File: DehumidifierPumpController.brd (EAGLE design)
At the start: 68.6 x 53.3 mm, 6 parts, among them P1 12V

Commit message: updated Picture and tinkercad sketch file
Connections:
- removed net N$4 (its old number): R4.2, U1.GND.
- removed net N$9 (its old number): K1.1, U1.GND
- new net N$2: K1.1, R4.2, U1.GND.
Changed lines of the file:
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@@
 <element value="" name="U1" library="AUTODESK_CIRCUITS_BREADBOARD" package="ARDUINO_UNO" x="5" y="10.08"></element><element value="" name="S1" library="AUTODESK_CIRCUITS_BREADBOARD" package="TL1105" x="5" y="22.78"></element><element value="" name="M1" library="AUTODESK_CIRCUITS_BREADBOARD" package="2P-2.54-65/35MIL" x="5" y="35.480000000000004"></element><element value="" name="K1" library="AUTODESK_CIRCUITS_BREADBOARD" package="M3XXH" x="5" y="48.18"></element><element value="1k‎Ω" name="R4" library="AUTODESK_CIRCUITS_BREADBOARD" package="0207/10" x="5" y="60.879999999999995"></element><element value="12V" name="P1" library="AUTODESK_CIRCUITS_BREADBOARD" package="2P-2.54-65/35MIL" x="5" y="73.58"></element></elements>
 <signals>
-<signal name="N$1"><contactref element="S1" pad="4"></contactref><contactref element="R4" pad="1"></contactref><wire x1="7.25" y1="19.53" x2="-0.08000000000000007" y2="60.879999999999995" width="0" layer="19" extent="1-1"></wire></signal><signal name="N$2"><contactref element="S1" pad="2"></contactref><contactref element="U1" pad="2"></contactref><wire x1="7.25" y1="26.03" x2="63.42" y2="60.879999999999995" width="0" layer="19" extent="1-1"></wire></signal><signal name="N$3"><contactref element="S1" pad="1"></contactref></signal><signal name="N$4"><contactref element="R4" pad="2"></contactref><contactref element="U1" pad="GND."></contactref><wire x1="10.08" y1="60.879999999999995" x2="48.18" y2="12.620000000000001" width="0" layer="19" extent="1-1"></wire></signal><signal name="N$5"><contactref element="K1" pad="2"></contactref><contactref element="U1" pad="7"></contactref><wire x1="1.19" y1="44.37" x2="50.72" y2="60.879999999999995" width="0" layer="19" extent="1-1"></wire></signal><signal name="N$6"><contactref element="M1" pad="1"></contactref><contactref element="P1" pad="1"></contactref><wire x1="5" y1="36.75000000000001" x2="5" y2="74.85" width="0" layer="19" extent="1-1"></wire></signal><signal name="N$7"><contactref element="P1" pad="2"></contactref><contactref element="K1" pad="P"></contactref><wire x1="5" y1="72.31" x2="11.35" y2="44.37" width="0" layer="19" extent="1-1"></wire></signal><signal name="N$8"><contactref element="K1" pad="S"></contactref><contactref element="M1" pad="2"></contactref><wire x1="-1.3499999999999996" y1="51.99" x2="5" y2="34.21" width="0" layer="19" extent="1-1"></wire></signal><signal name="N$9"><contactref element="U1" pad="GND"></contactref><contactref element="K1" pad="1"></contactref><wire x1="31.416" y1="60.879999999999995" x2="1.19" y2="51.99" width="0" layer="19" extent="1-1"></wire></signal><signal name="N$10"><contactref element="U1" pad="5V"></contactref><contactref element="S1" pad="3"></contactref><wire x1="43.1" y1="12.620000000000001" x2="2.75" y2="19.53" width="0" layer="19" extent="1-1"></wire></signal></signals>
+<signal name="N$1"><contactref element="S1" pad="4"></contactref><contactref element="R4" pad="1"></contactref><wire x1="7.25" y1="19.53" x2="-0.08000000000000007" y2="60.879999999999995" width="0" layer="19" extent="1-1"></wire></signal><signal name="N$2"><contactref element="U1" pad="GND."></contactref><contactref element="K1" pad="1"></contactref><wire x1="48.18" y1="12.620000000000001" x2="1.19" y2="51.99" width="0" layer="19" extent="1-1"></wire><contactref element="R4" pad="2"></contactref><wire x1="1.19" y1="51.99" x2="10.08" y2="60.879999999999995" width="0" layer="19" extent="1-1"></wire></signal><signal name="N$3"><contactref element="M1" pad="1"></contactref><contactref element="P1" pad="1"></contactref><wire x1="5" y1="36.75000000000001" x2="5" y2="74.85" width="0" layer="19" extent="1-1"></wire></signal><signal name="N$4"><contactref element="U1" pad="5V"></contactref><contactref element="S1" pad="3"></contactref><wire x1="43.1" y1="12.620000000000001" x2="2.75" y2="19.53" width="0" layer="19" extent="1-1"></wire></signal><signal name="N$5"><contactref element="U1" pad="2"></contactref><contactref element="S1" pad="2"></contactref><wire x1="63.42" y1="60.879999999999995" x2="7.25" y2="26.03" width="0" layer="19" extent="1-1"></wire></signal><signal name="N$6"><contactref element="S1" pad="1"></contactref></signal><signal name="N$7"><contactref element="K1" pad="P"></contactref><contactref element="P1" pad="2"></contactref><wire x1="11.35" y1="44.37" x2="5" y2="72.31" width="0" layer="19" extent="1-1"></wire></signal><signal name="N$8"><contactref element="U1" pad="7"></contactref><contactref element="K1" pad="2"></contactref><wire x1="50.72" y1="60.879999999999995" x2="1.19" y2="44.37" width="0" layer="19" extent="1-1"></wire></signal><signal name="N$9"><contactref element="K1" pad="S"></contactref><contactref element="M1" pad="2"></contactref><wire x1="-1.3499999999999996" y1="51.99" x2="5" y2="34.21" width="0" layer="19" extent="1-1"></wire></signal></signals>
 </board>
 </drawing>

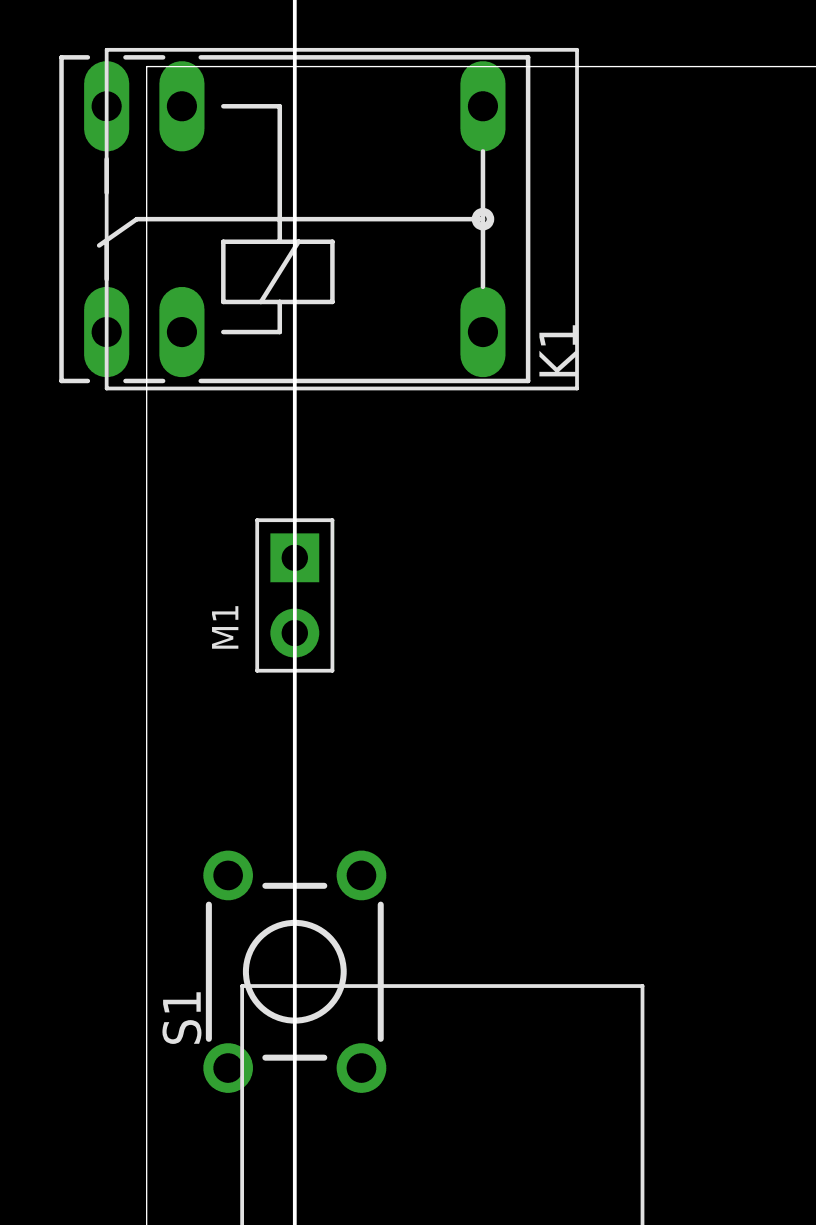
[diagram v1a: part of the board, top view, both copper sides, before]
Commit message: updated some files
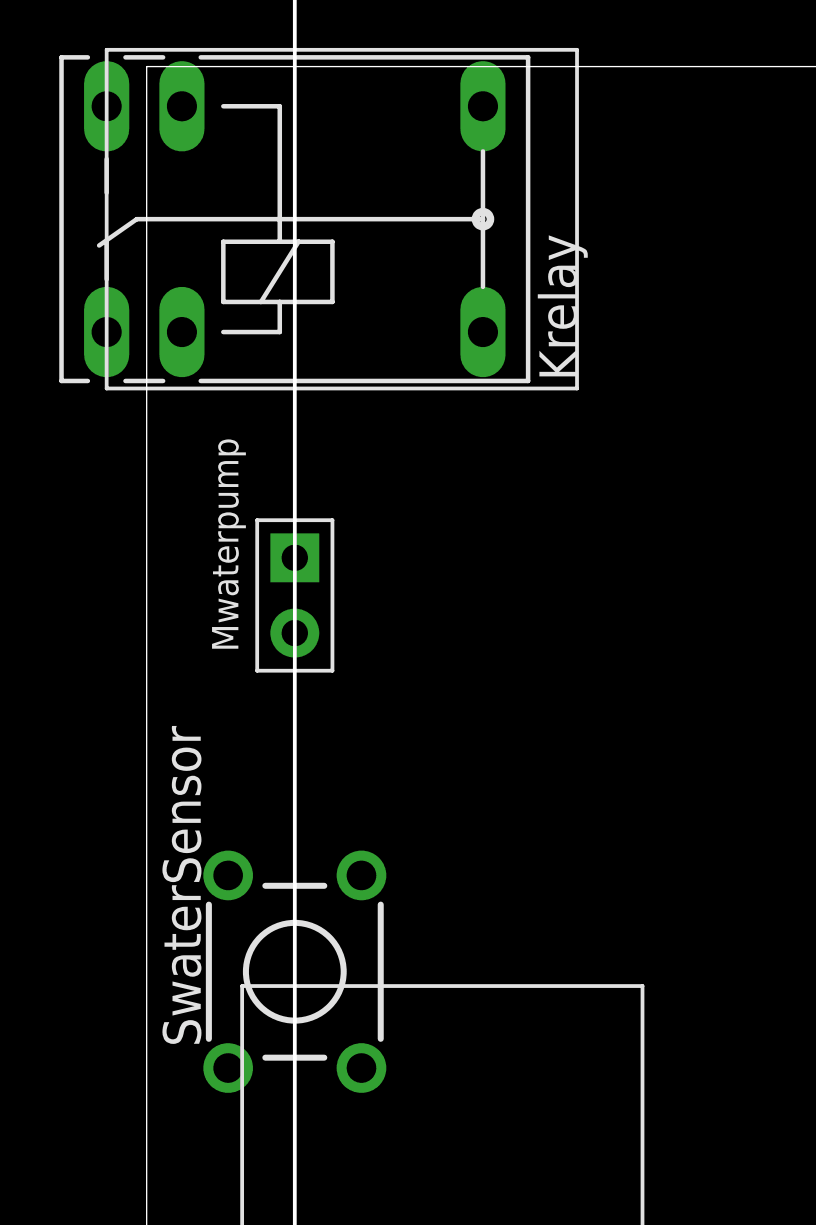
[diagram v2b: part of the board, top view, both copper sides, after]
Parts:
- renumbered K1 to Krelay, M1 to Mwaterpump, S1 to SwaterSensor
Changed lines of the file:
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@@
 </autorouter>
 <elements>
-<element value="" name="U1" library="AUTODESK_CIRCUITS_BREADBOARD" package="ARDUINO_UNO" x="5" y="10.08"></element><element value="" name="S1" library="AUTODESK_CIRCUITS_BREADBOARD" package="TL1105" x="5" y="22.78"></element><element value="" name="M1" library="AUTODESK_CIRCUITS_BREADBOARD" package="2P-2.54-65/35MIL" x="5" y="35.480000000000004"></element><element value="" name="K1" library="AUTODESK_CIRCUITS_BREADBOARD" package="M3XXH" x="5" y="48.18"></element><element value="1k‎Ω" name="R4" library="AUTODESK_CIRCUITS_BREADBOARD" package="0207/10" x="5" y="60.879999999999995"></element><element value="12V" name="P1" library="AUTODESK_CIRCUITS_BREADBOARD" package="2P-2.54-65/35MIL" x="5" y="73.58"></element></elements>
+<element value="" name="U1" library="AUTODESK_CIRCUITS_BREADBOARD" package="ARDUINO_UNO" x="5" y="10.08"></element><element value="" name="SwaterSensor" library="AUTODESK_CIRCUITS_BREADBOARD" package="TL1105" x="5" y="22.78"></element><element value="" name="Mwaterpump" library="AUTODESK_CIRCUITS_BREADBOARD" package="2P-2.54-65/35MIL" x="5" y="35.480000000000004"></element><element value="" name="Krelay" library="AUTODESK_CIRCUITS_BREADBOARD" package="M3XXH" x="5" y="48.18"></element><element value="1k‎Ω" name="R4" library="AUTODESK_CIRCUITS_BREADBOARD" package="0207/10" x="5" y="60.879999999999995"></element><element value="12V" name="P1" library="AUTODESK_CIRCUITS_BREADBOARD" package="2P-2.54-65/35MIL" x="5" y="73.58"></element></elements>
 <signals>
-<signal name="N$1"><contactref element="S1" pad="4"></contactref><contactref element="R4" pad="1"></contactref><wire x1="7.25" y1="19.53" x2="-0.08000000000000007" y2="60.879999999999995" width="0" layer="19" extent="1-1"></wire></signal><signal name="N$2"><contactref element="U1" pad="GND."></contactref><contactref element="K1" pad="1"></contactref><wire x1="48.18" y1="12.620000000000001" x2="1.19" y2="51.99" width="0" layer="19" extent="1-1"></wire><contactref element="R4" pad="2"></contactref><wire x1="1.19" y1="51.99" x2="10.08" y2="60.879999999999995" width="0" layer="19" extent="1-1"></wire></signal><signal name="N$3"><contactref element="M1" pad="1"></contactref><contactref element="P1" pad="1"></contactref><wire x1="5" y1="36.75000000000001" x2="5" y2="74.85" width="0" layer="19" extent="1-1"></wire></signal><signal name="N$4"><contactref element="U1" pad="5V"></contactref><contactref element="S1" pad="3"></contactref><wire x1="43.1" y1="12.620000000000001" x2="2.75" y2="19.53" width="0" layer="19" extent="1-1"></wire></signal><signal name="N$5"><contactref element="U1" pad="2"></contactref><contactref element="S1" pad="2"></contactref><wire x1="63.42" y1="60.879999999999995" x2="7.25" y2="26.03" width="0" layer="19" extent="1-1"></wire></signal><signal name="N$6"><contactref element="S1" pad="1"></contactref></signal><signal name="N$7"><contactref element="K1" pad="P"></contactref><contactref element="P1" pad="2"></contactref><wire x1="11.35" y1="44.37" x2="5" y2="72.31" width="0" layer="19" extent="1-1"></wire></signal><signal name="N$8"><contactref element="U1" pad="7"></contactref><contactref element="K1" pad="2"></contactref><wire x1="50.72" y1="60.879999999999995" x2="1.19" y2="44.37" width="0" layer="19" extent="1-1"></wire></signal><signal name="N$9"><contactref element="K1" pad="S"></contactref><contactref element="M1" pad="2"></contactref><wire x1="-1.3499999999999996" y1="51.99" x2="5" y2="34.21" width="0" layer="19" extent="1-1"></wire></signal></signals>
+<signal name="N$1"><contactref element="Mwaterpump" pad="1"></contactref><contactref element="P1" pad="1"></contactref><wire x1="5" y1="36.75000000000001" x2="5" y2="74.85" width="0" layer="19" extent="1-1"></wire></signal><signal name="N$2"><contactref element="U1" pad="5V"></contactref><contactref element="SwaterSensor" pad="3"></contactref><wire x1="43.1" y1="12.620000000000001" x2="2.75" y2="19.53" width="0" layer="19" extent="1-1"></wire></signal><signal name="N$3"><contactref element="Krelay" pad="P"></contactref><contactref element="P1" pad="2"></contactref><wire x1="11.35" y1="44.37" x2="5" y2="72.31" width="0" layer="19" extent="1-1"></wire></signal><signal name="N$4"><contactref element="U1" pad="7"></contactref><contactref element="Krelay" pad="2"></contactref><wire x1="50.72" y1="60.879999999999995" x2="1.19" y2="44.37" width="0" layer="19" extent="1-1"></wire></signal><signal name="N$5"><contactref element="Krelay" pad="S"></contactref><contactref element="Mwaterpump" pad="2"></contactref><wire x1="-1.3499999999999996" y1="51.99" x2="5" y2="34.21" width="0" layer="19" extent="1-1"></wire></signal><signal name="N$6"><contactref element="SwaterSensor" pad="4"></contactref><contactref element="R4" pad="1"></contactref><wire x1="7.25" y1="19.53" x2="-0.08000000000000007" y2="60.879999999999995" width="0" layer="19" extent="1-1"></wire></signal><signal name="N$7"><contactref element="SwaterSensor" pad="2"></contactref><contactref element="U1" pad="2"></contactref><wire x1="7.25" y1="26.03" x2="63.42" y2="60.879999999999995" width="0" layer="19" extent="1-1"></wire></signal><signal name="N$8"><contactref element="SwaterSensor" pad="1"></contactref></signal><signal name="N$9"><contactref element="R4" pad="2"></contactref><contactref element="U1" pad="GND."></contactref><wire x1="10.08" y1="60.879999999999995" x2="48.18" y2="12.620000000000001" width="0" layer="19" extent="1-1"></wire><contactref element="Krelay" pad="1"></contactref><wire x1="48.18" y1="12.620000000000001" x2="1.19" y2="51.99" width="0" layer="19" extent="1-1"></wire></signal></signals>
 </board>
 </drawing>
